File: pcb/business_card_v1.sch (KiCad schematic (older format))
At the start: 68 parts, among them J1 Conn_01x05_Male, J2 Conn_01x01_Male, SW1 SW_SPST, U1 MIC5504-3.3YM5, U2 STM32G030F6P6

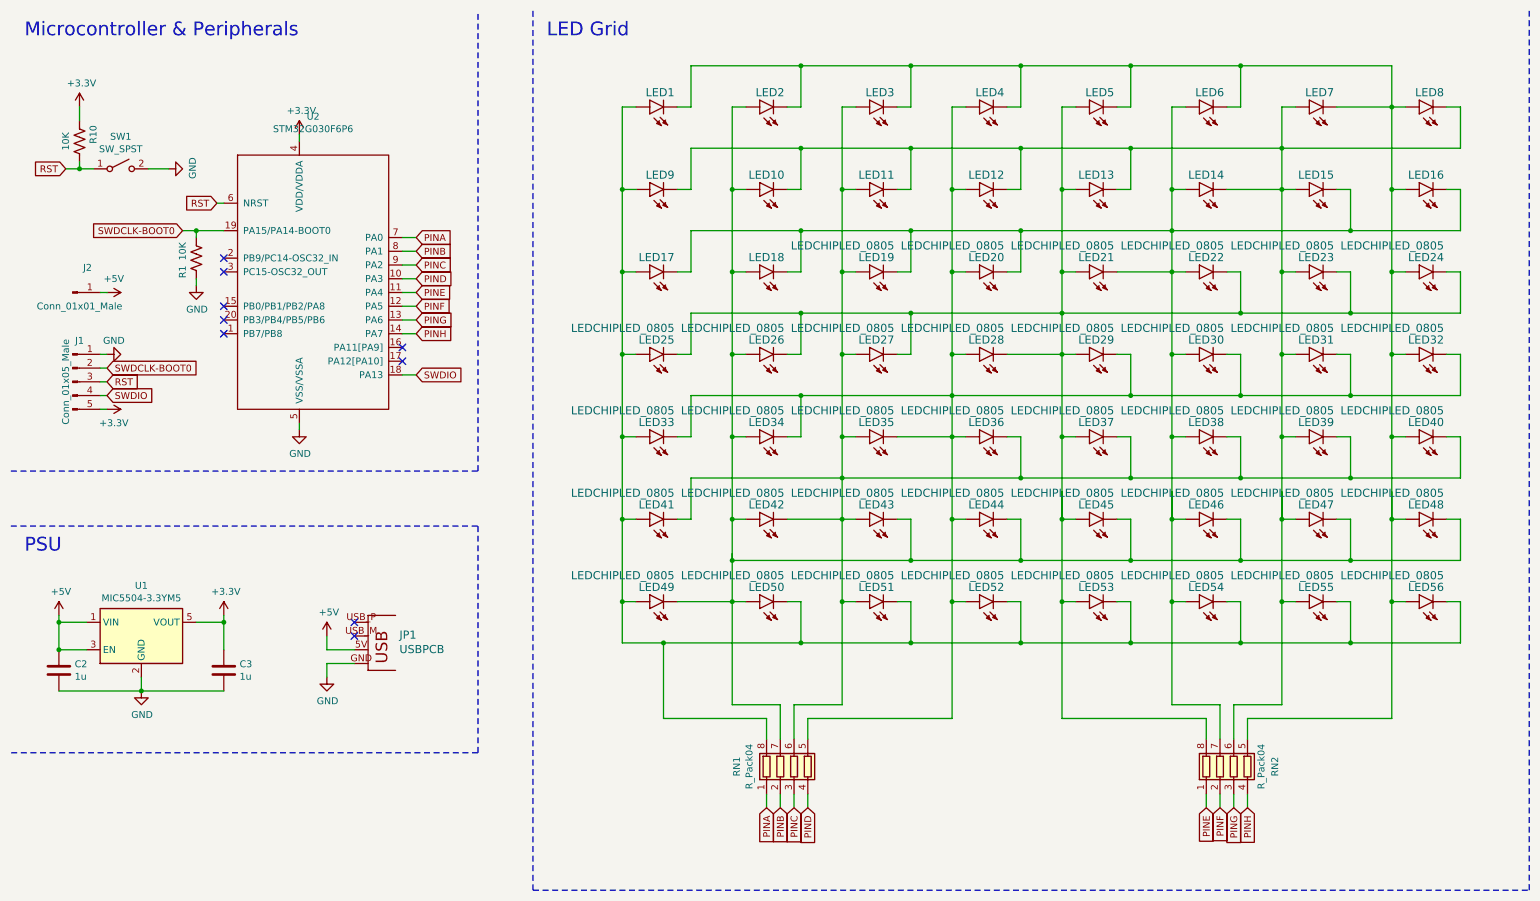
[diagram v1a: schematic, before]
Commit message: update card to v4
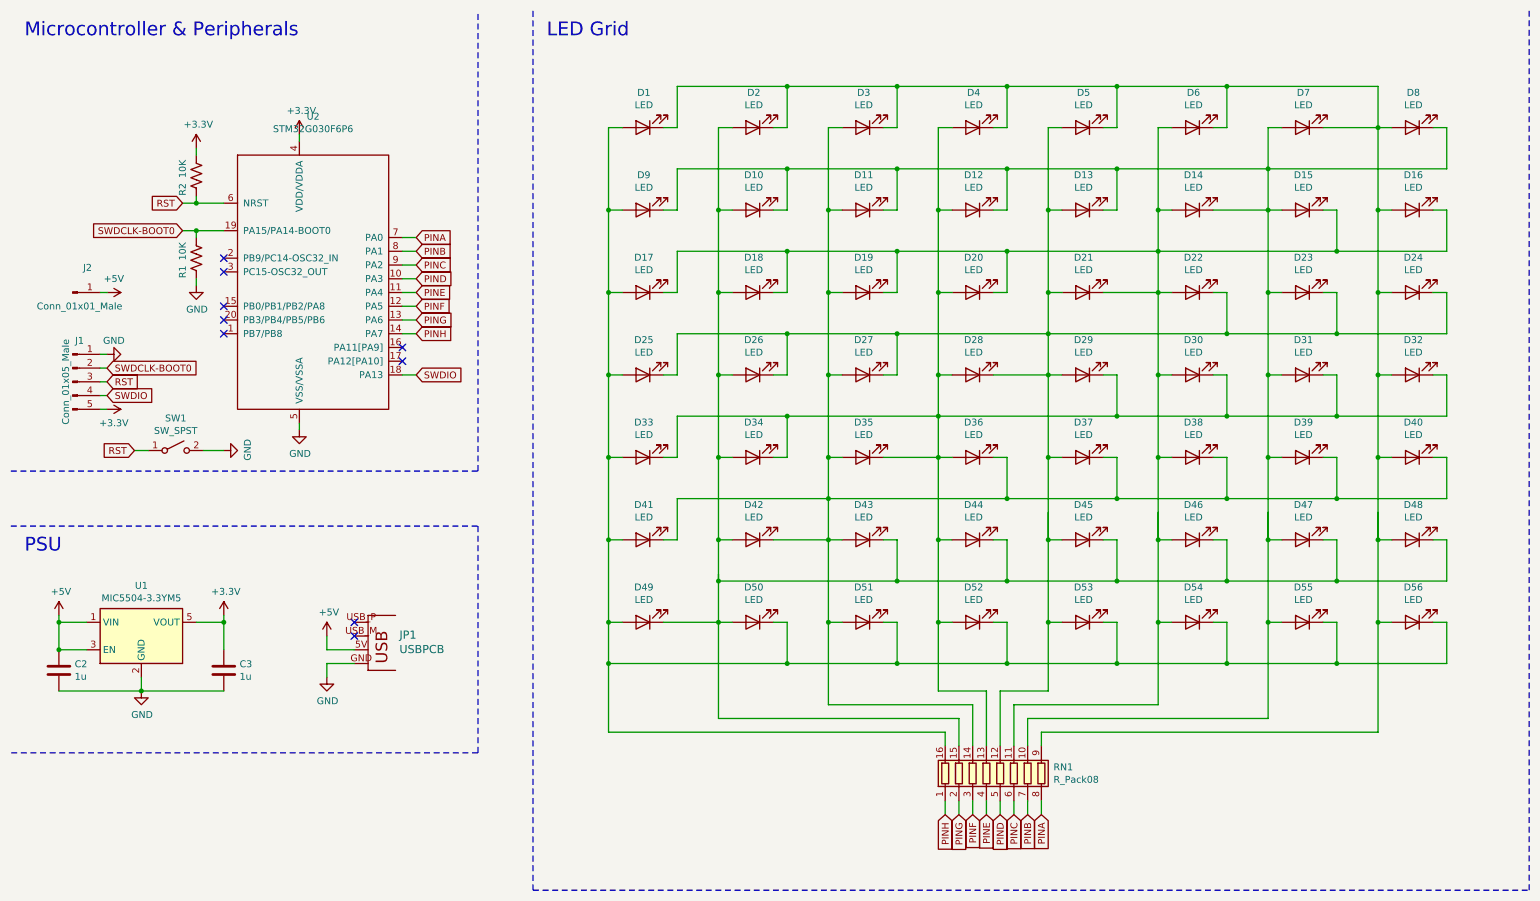
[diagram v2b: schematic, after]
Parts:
- removed LED1, LED10, LED11, LED12, LED13, LED14, LED15, LED16, LED17, LED18, LED19, LED2, LED20, LED21, LED22, LED23, LED24, LED25, LED26, LED27, LED28, LED29, LED3, LED30, LED31, LED32, LED33, LED34, LED35, LED36, LED37, LED38, LED39, LED4, LED40, LED41, LED42, LED43, LED44, LED45, LED46, LED47, LED48, LED49, LED5, LED50, LED51, LED52, LED53, LED54, LED55, LED56, LED6, LED7, LED8, LED9: LEDCHIPLED_0805, business_card_v1:CHIPLED_0805, symbol business_card_v1-eagle-import:LEDCHIPLED_0805
- removed R10: 10K, Resistor_SMD:R_0603_1608Metric, symbol Device:R_US
- removed RN1, RN2: R_Pack04, Resistor_SMD:R_Array_Convex_4x0603, symbol Device:R_Pack04
- added D1, D10, D11, D12, D13, D14, D15, D16, D17, D18, D19, D2, D20, D21, D22, D23, D24, D25, D26, D27, D28, D29, D3, D30, D31, D32, D33, D34, D35, D36, D37, D38, D39, D4, D40, D41, D42, D43, D44, D45, D46, D47, D48, D49, D5, D50, D51, D52, D53, D54, D55, D56, D6, D7, D8, D9: LED, Resistor_SMD:R_0805_2012Metric, symbol Device:LED
- added R2: 10K, Resistor_SMD:R_0603_1608Metric, symbol Device:R_US
- added RN1: R_Pack08, Resistor_SMD:R_Array_Convex_8x0602, symbol Device:R_Pack08
- J2: footprint Connector_PinSocket_2.54mm:PinSocket_1x01_P2.54mm_Vertical -> Connector_PinHeader_2.54mm:PinHeader_1x01_P2.54mm_Vertical
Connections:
- net +3V3: now also R2.1
- net PINA: now also RN1.8 (R8.1)
- net PINB: now also RN1.7 (R7.1)
- net PINC: now also RN1.6 (R6.1)
- net PIND: now also RN1.5 (R5.1)
- net PINE: now also RN1.4 (R4.1)
- net PINF: now also RN1.3 (R3.1)
- net PING: now also RN1.2 (R2.1)
- net PINH: now also RN1.1 (R1.1)
- net RST: now also R2.2
- new net: D10.1 (K), D11.1 (K), D12.1 (K), D13.1 (K), D14.1 (K), D15.2 (A), D23.2 (A), D31.2 (A), D39.2 (A), D47.2 (A), D55.2 (A), D7.2 (A), D8.1 (K), D9.1 (K), RN1.10 (R7.2)
- new net: D14.2 (A), D15.1 (K), D16.1 (K), D17.1 (K), D18.1 (K), D19.1 (K), D20.1 (K), D21.1 (K), D22.2 (A), D30.2 (A), D38.2 (A), D46.2 (A), D54.2 (A), D6.2 (A), RN1.11 (R6.2)
- new net: D13.2 (A), D21.2 (A), D22.1 (K), D23.1 (K), D24.1 (K), D25.1 (K), D26.1 (K), D27.1 (K), D28.1 (K), D29.2 (A), D37.2 (A), D45.2 (A), D5.2 (A), D53.2 (A), RN1.12 (R5.2)
- new net: D12.2 (A), D20.2 (A), D28.2 (A), D29.1 (K), D30.1 (K), D31.1 (K), D32.1 (K), D33.1 (K), D34.1 (K), D35.1 (K), D36.2 (A), D4.2 (A), D44.2 (A), D52.2 (A), RN1.13 (R4.2)
- new net: D11.2 (A), D19.2 (A), D27.2 (A), D3.2 (A), D35.2 (A), D36.1 (K), D37.1 (K), D38.1 (K), D39.1 (K), D40.1 (K), D41.1 (K), D42.1 (K), D43.2 (A), D51.2 (A), RN1.14 (R3.2)
- new net: D10.2 (A), D18.2 (A), D2.2 (A), D26.2 (A), D34.2 (A), D42.2 (A), D43.1 (K), D44.1 (K), D45.1 (K), D46.1 (K), D47.1 (K), D48.1 (K), D49.1 (K), D50.2 (A), RN1.15 (R2.2)
- new net: D1.2 (A), D17.2 (A), D25.2 (A), D33.2 (A), D41.2 (A), D49.2 (A), D50.1 (K), D51.1 (K), D52.1 (K), D53.1 (K), D54.1 (K), D55.1 (K), D56.1 (K), D9.2 (A), RN1.16 (R1.2)
- new net: D1.1 (K), D16.2 (A), D2.1 (K), D24.2 (A), D3.1 (K), D32.2 (A), D4.1 (K), D40.2 (A), D48.2 (A), D5.1 (K), D56.2 (A), D6.1 (K), D7.1 (K), D8.2 (A), RN1.9 (R8.2)
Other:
- moved on the sheet: SW1
